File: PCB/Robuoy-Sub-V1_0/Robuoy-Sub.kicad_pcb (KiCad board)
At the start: 4 copper layers, 160 x 160 mm, 142 parts, among them J101 PROG/JTAG, J102 PUSH BUTTON, J103 ESC_BB, J104 ESC_SB, J105 RS232_Option, J106 Compass, J201 Accu, J202 LoadbalanceAccu1, J203 LoadbalanceAccu2, J204 CHARGE/ON-OFF, J205 PWR_Charger, J206 LoadbalanceCharger, J207 ESCSB, J208 ESCBB, Q101 AO3400A, Q102 AO3400A, Q201 AO3400A, Q202 AO3400A, Q203 AO3400A, Q204 AO3400A, Q205 AO3400A, Q206 AO3400A, Q207 AO3400A, Q208 AO3400A, SW101 ~{BOOT}, SW102 ~{RESET}, SW201 On/Off, U101 ESP32-WROOM-32E_(visible_peri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, U102 USBLC6-4SC6, U103 LTC4311, U104 SN74LV1T34DBV, U105 SN74LV1T34DBV, U106 LSM303AGRTR, U201 TPS5430DDAR, U202 SN74LV1T34DBV, U203 SN74LV1T34DBV, U204 TLV61046ADB

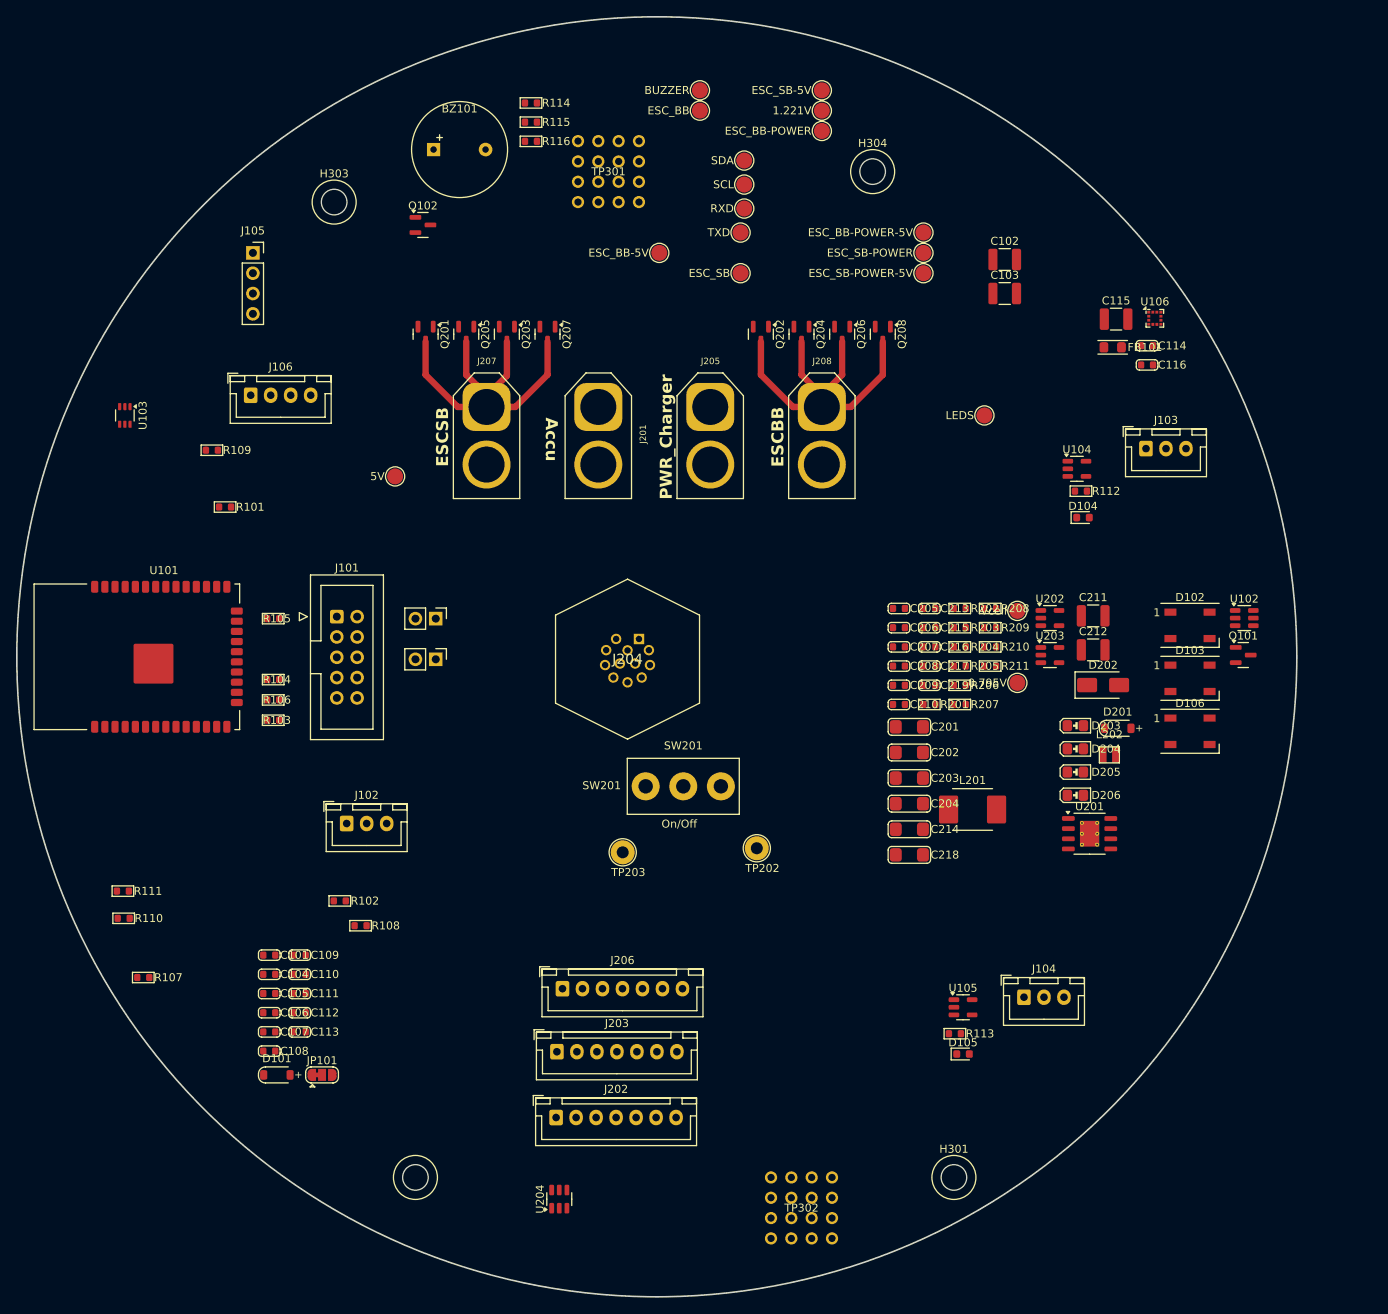
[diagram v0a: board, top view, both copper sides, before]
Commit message: Pcb edditing
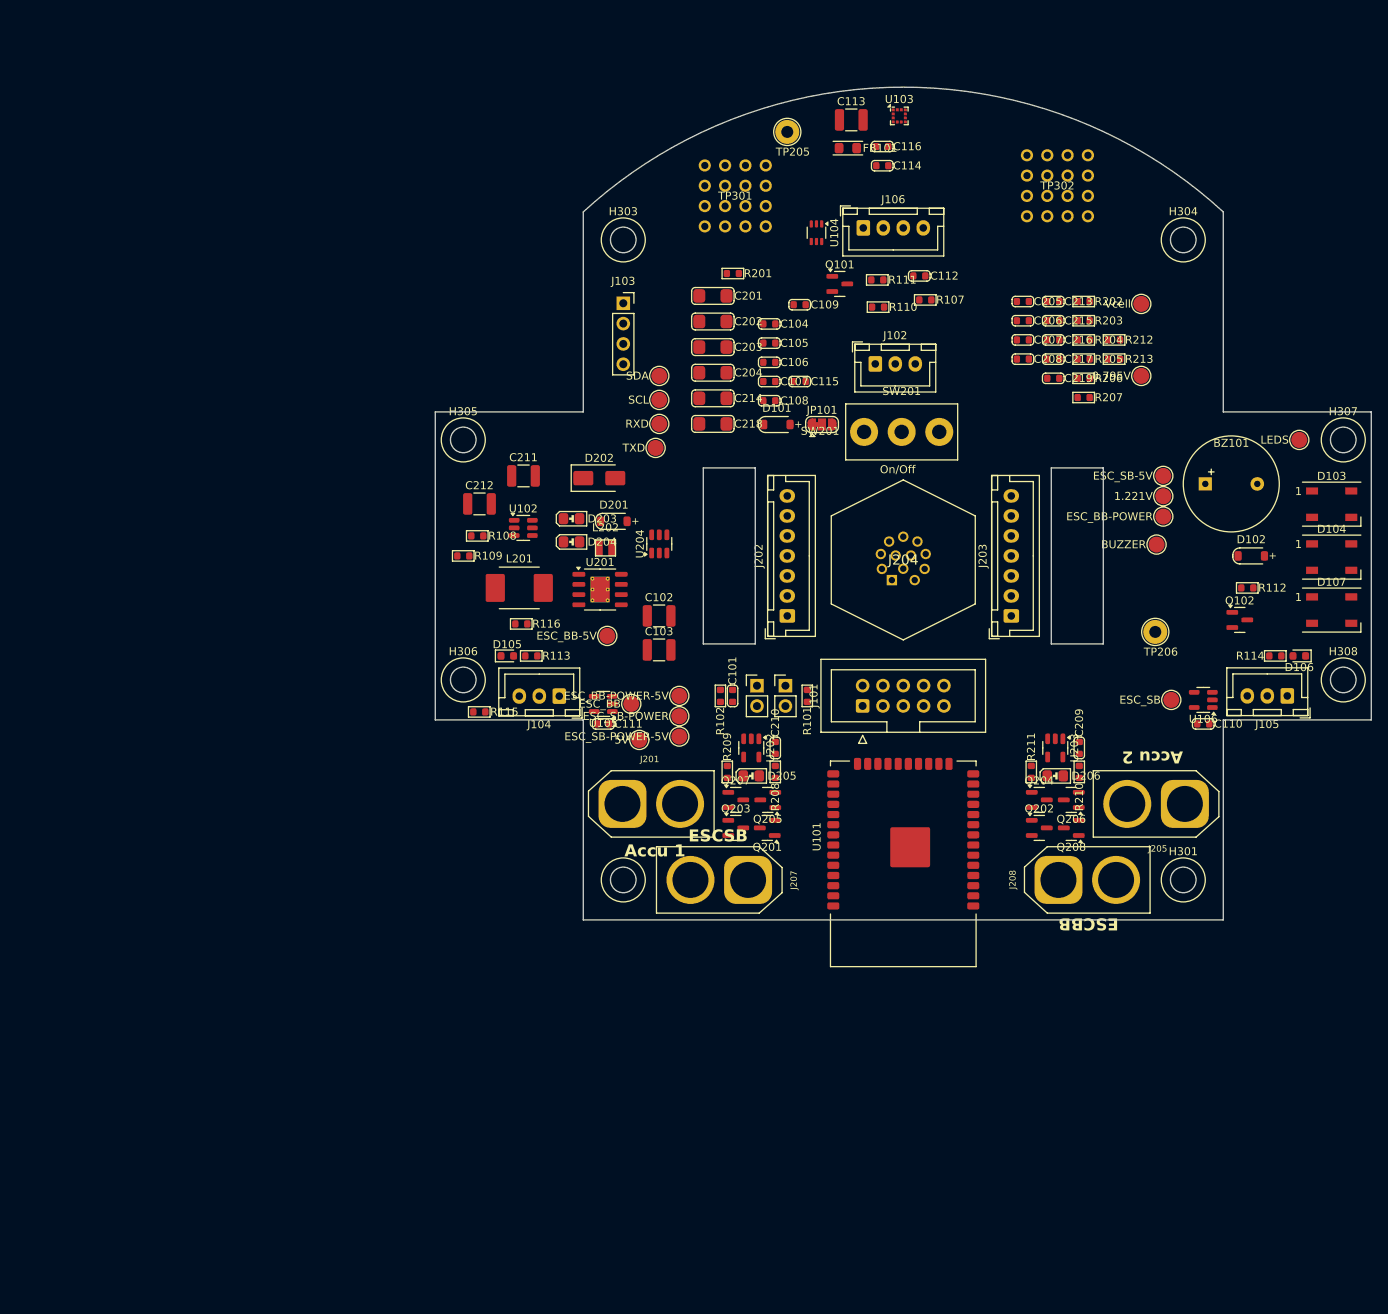
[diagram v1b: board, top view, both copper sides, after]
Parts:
- removed J206: LoadbalanceCharger, Connector_JST:JST_XH_B7B-XH-A_1x07_P2.50mm_Vertical
- removed R103, R104, R105, R106: 100, A_Device:R_0603
- added D102: SM4007PL, A_Device:D_SOD-123_2.85x1.8x1.3, F.Cu at (169.3, 97.4)
- added H305: MountingHole, A_Mechanical:NPTH_M3, F.Cu at (70.8, 82.9)
- added H306: MountingHole, A_Mechanical:NPTH_M3, F.Cu at (70.8, 112.9)
- added H307: MountingHole, A_Mechanical:NPTH_M3, F.Cu at (180.8, 82.9)
- added H308: MountingHole, A_Mechanical:NPTH_M3, F.Cu at (180.8, 112.9)
- added R209: 100, A_Device:R_0603, F.Cu at (103.8, 124.4)
- added R211: 100, A_Device:R_0603, F.Cu at (141.8, 124.4)
- J201: value Accu -> Accu 1
- J205: value PWR_Charger -> Accu 2; footprint A_Connector:AMASS_XT60-F_1x02_P7.20mm_Vertical -> A_Connector:AMASS_XT60-M_1x02_P7.20mm_Vertical
- moved TP302 131.7 mm to (145.1, 51.1)
- moved R107 129.3 mm to (128.6, 65.4)
- moved R110 121.4 mm to (122.7, 66.3)
- moved R111 121.4 mm to (122.6, 62.9)
- moved C112 120.3 mm to (127.8, 62.4)
- moved C110 117.2 mm to (163.3, 118.4)
- moved Q102 113.4 mm to (167.9, 105.4)
- moved R112 105.5 mm to (168.8, 101.4)
- moved BZ101 105.1 mm to (166.8, 88.4)
- moved C104 102.5 mm to (109.1, 68.4)
- moved C105 102.5 mm to (109.1, 70.8)
- moved C106 102.5 mm to (109.1, 73.2)
- moved C108 102.5 mm to (109.1, 78.0)
- moved C109 102.5 mm to (112.9, 66.0)
- moved C107 102.5 mm to (109.1, 75.6)
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- renumbered C115 to C113, C116 to C114, C113 to C115, C114 to C116, D102 to D103, D103 to D104, D104 to D105, D105 to D106, D106 to D107, J105 to J103, J103 to J104, J104 to J105, R116 to R112, R112 to R113, R113 to R114, R114 to R115, R115 to R116, R209 to R210, R210 to R212, R211 to R213, TP109 to TP102, TP110 to TP103, TP108 to TP104, TP107 to TP105, TP104 to TP106, TP102 to TP107, TP103 to TP108, TP105 to TP109, TP106 to TP110, TP206 to TP202, TP208 to TP203, TP207 to TP204, TP202 to TP205, TP203 to TP206, TP210 to TP207, TP209 to TP208, TP204 to TP209, TP205 to TP210, U106 to U103, U103 to U104, U104 to U105, U105 to U106
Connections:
- J101 pad 10: Net-(J101-Pin_10) -> MTDI
- J101 pad 7: Net-(J101-Pin_7) -> MTMS
- J101 pad 8: Net-(J101-Pin_8) -> MTCK
- J101 pad 9: Net-(J101-Pin_9) -> MTDO
- J204 pad 1: Net-(J202-Pin_1) -> Vbatt
- J204 pad 10: GND -> Net-(J202-Pin_3)
- J204 pad 11: Vbatt -> Net-(J202-Pin_2)
- J204 pad 12: Vbatt -> Net-(J202-Pin_1)
- J204 pad 2: Net-(J202-Pin_2) -> Vbatt
- J204 pad 3: Net-(J202-Pin_3) -> GND
- J204 pad 4: Net-(J202-Pin_4) -> GND
- J204 pad 5: Net-(J202-Pin_5) -> +VSW
- J204 pad 6: Net-(J202-Pin_6) -> Net-(J202-Pin_7)
- J204 pad 7: Net-(J202-Pin_7) -> Net-(J202-Pin_6)
- J204 pad 8: +VSW -> Net-(J202-Pin_5)
- J204 pad 9: GND -> Net-(J202-Pin_4)
- U202 pad 4: Net-(Q201-G) -> Net-(U202-Y)
- U203 pad 4: Net-(Q202-G) -> Net-(U203-Y)
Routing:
- net Net-(D205-K): track 45.3 -> 0.00 mm
- net Net-(D206-K): track 43.8 -> 0.00 mm
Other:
- board size 160 x 160 mm -> 117 x 104.1 mm
